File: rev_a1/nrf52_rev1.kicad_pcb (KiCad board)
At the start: 2 copper layers, 48.3 x 48.3 mm, 31 parts, among them P1 CONN_01X18, P2 CONN_01X18, P3 USB_OTG, U1 nRF52832, U2 CP2102, U3 LT1129CST-3.3, Y1 32K, Y2 32M

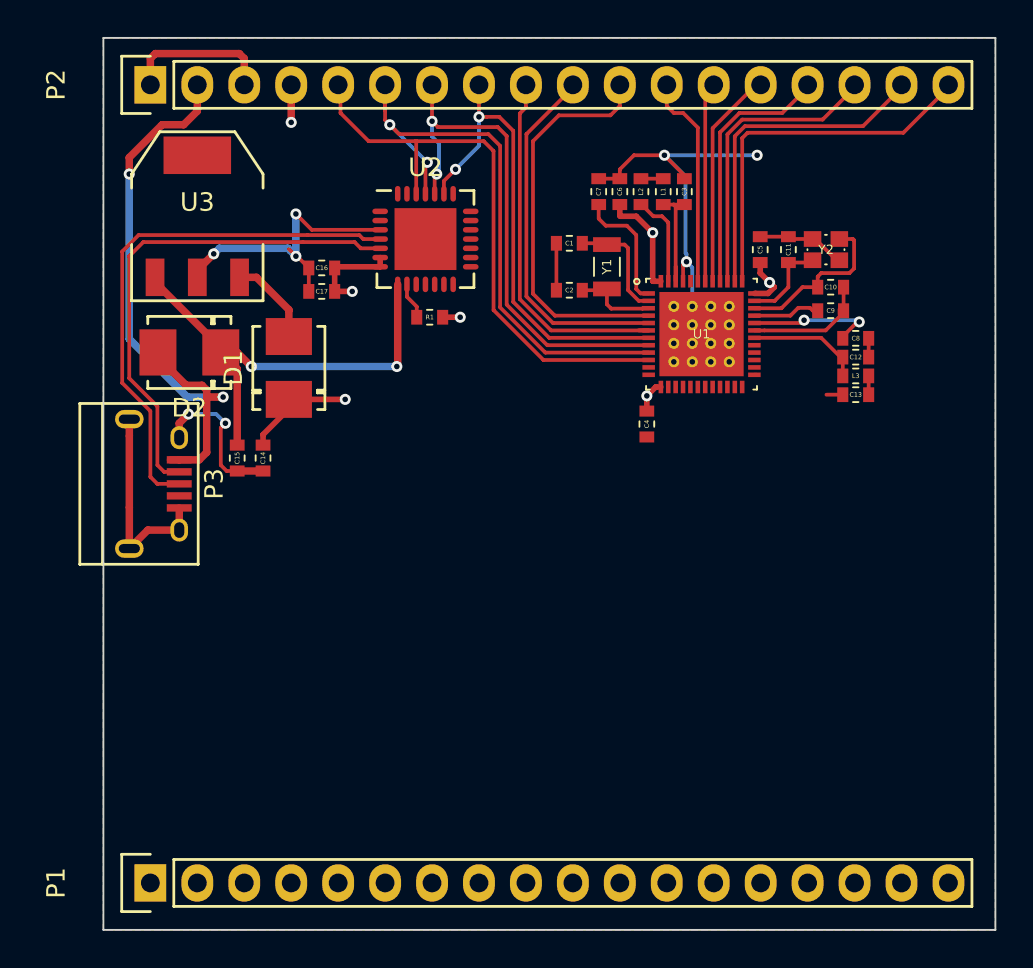
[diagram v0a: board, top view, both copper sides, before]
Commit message: Added logo etc
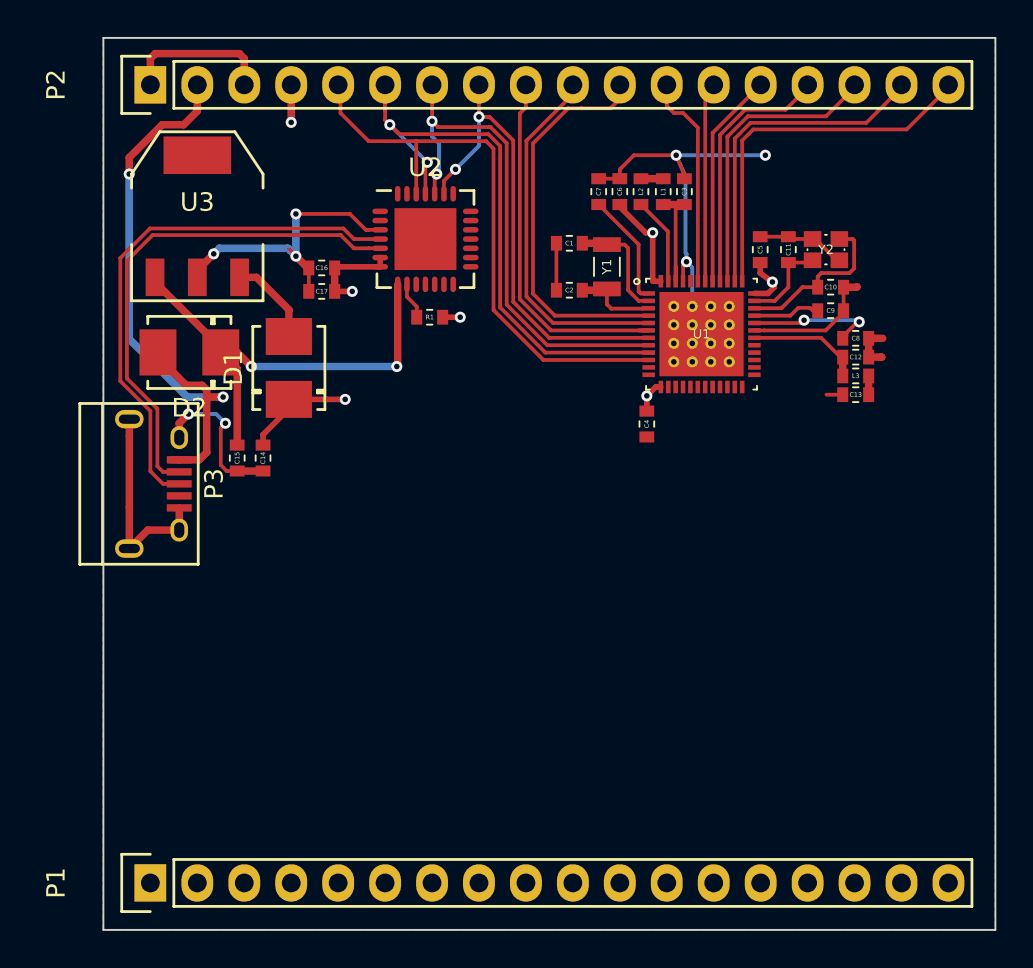
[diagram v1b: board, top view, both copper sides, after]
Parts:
- added G***: LOGO, xil_assets:logo_inv, B.Cu at (50.8, 49.5)
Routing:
- net GND: track 115.2 -> 117.2 mm
- net Net-(L1-Pad1): track 1.27 -> 2.48 mm
- net Net-(C3-Pad1): track 6.13 -> 7.28 mm
- net Net-(C7-Pad1): track 6.85 -> 6.18 mm
